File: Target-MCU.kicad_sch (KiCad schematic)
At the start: 25 parts, among them Q3 DMG1012UW-7, SW4 SKRPASE010

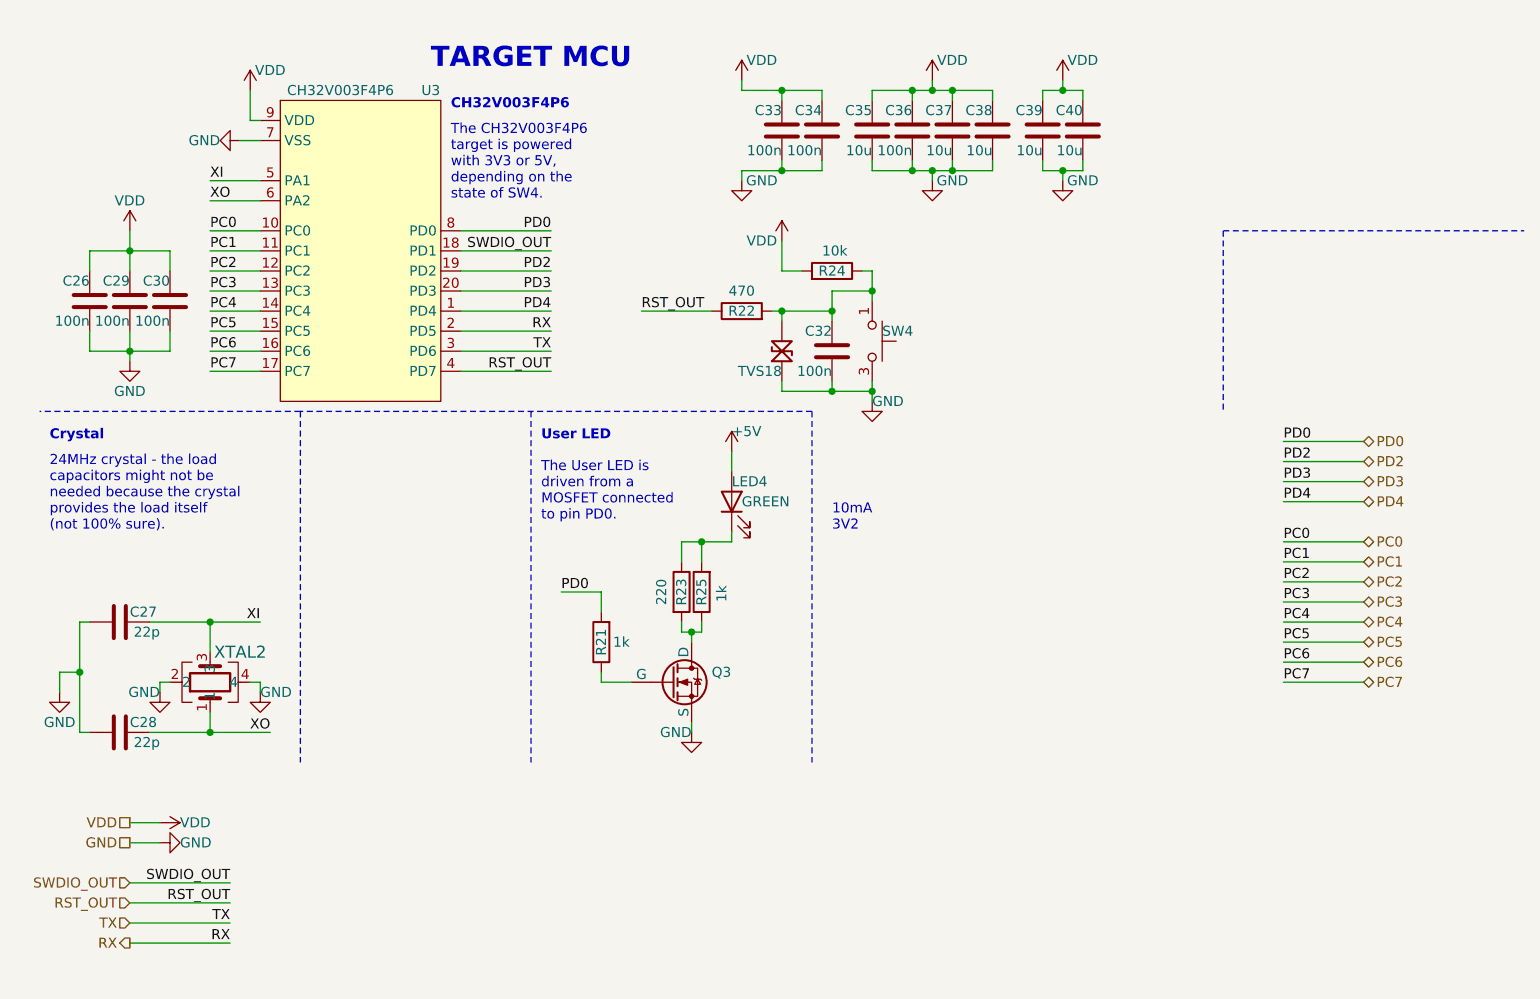
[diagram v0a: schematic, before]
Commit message: Update schematic
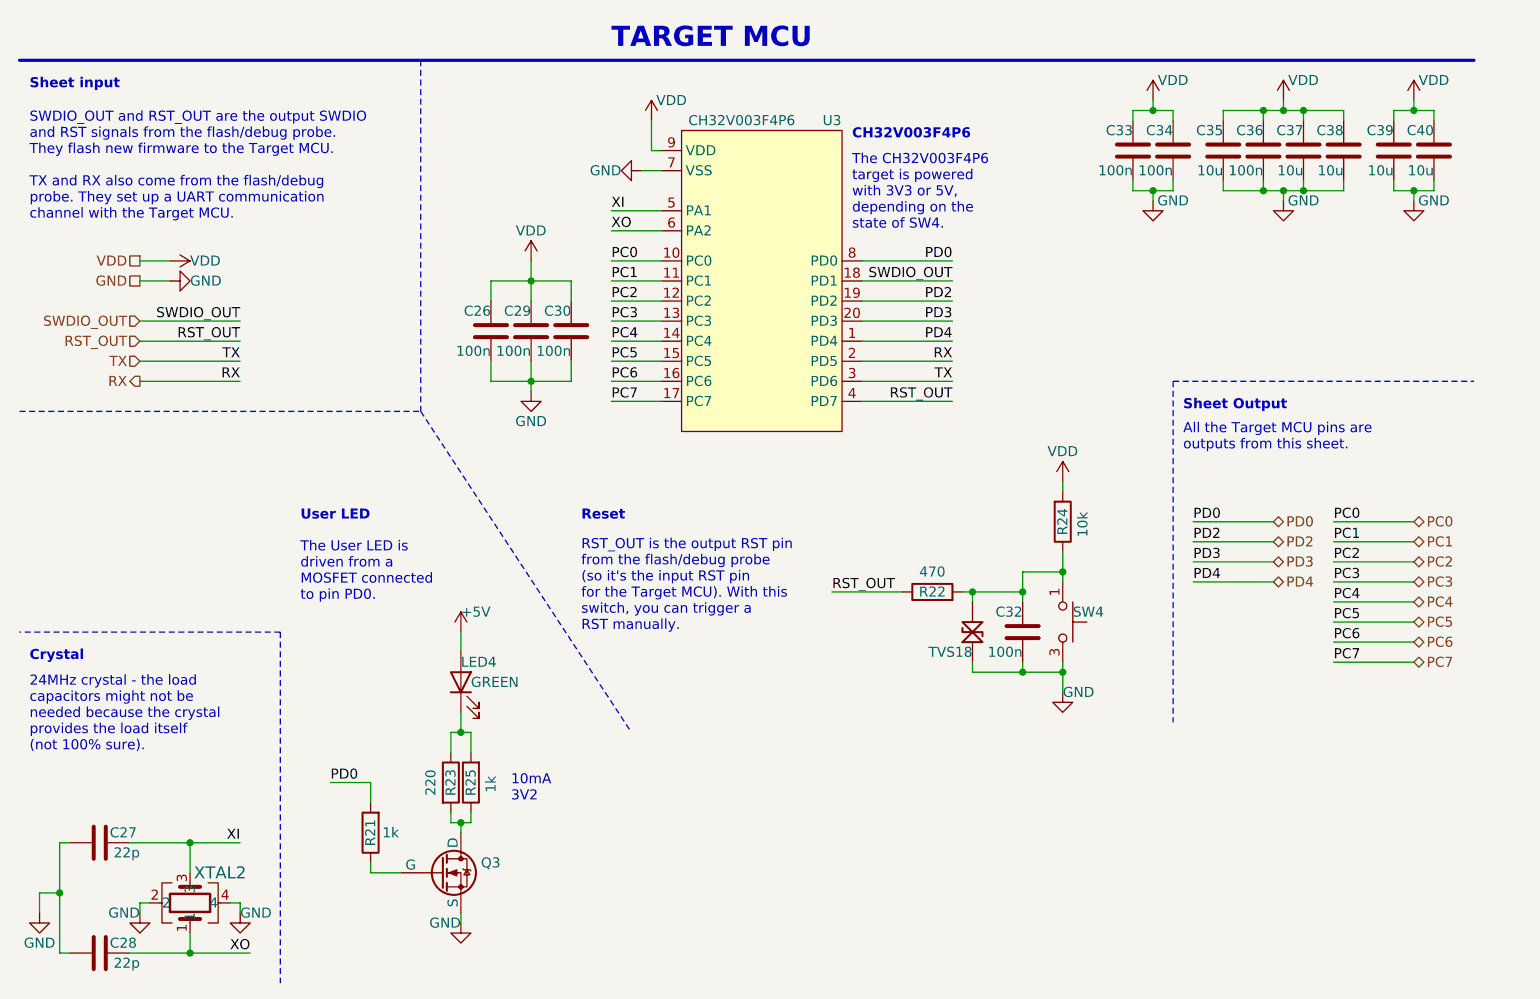
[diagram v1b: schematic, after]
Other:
- note added: "All the Target MCU pins are outputs from this sheet."
- note added: "RST_OUT is the output RST pin from the flash/debug probe (so it's the input RST pin for the Target MCU). With this switch, you can trigger a RST manually."
- note added: "Reset"
- note added: "SWDIO_OUT and RST_OUT are the output SWDIO and RST signals from the flash/debug probe. They flash new firmware to the Target MCU. TX and RX also come from the flash/debug probe. They set up a UART communication channel with the Target MCU."
- note added: "Sheet Output"
- note added: "Sheet input"
- moved on the sheet: C26, C27, C28, C29, C30, C32, C33, C34, C35, C36, C37, C38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
